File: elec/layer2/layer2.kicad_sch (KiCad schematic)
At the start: 19 parts

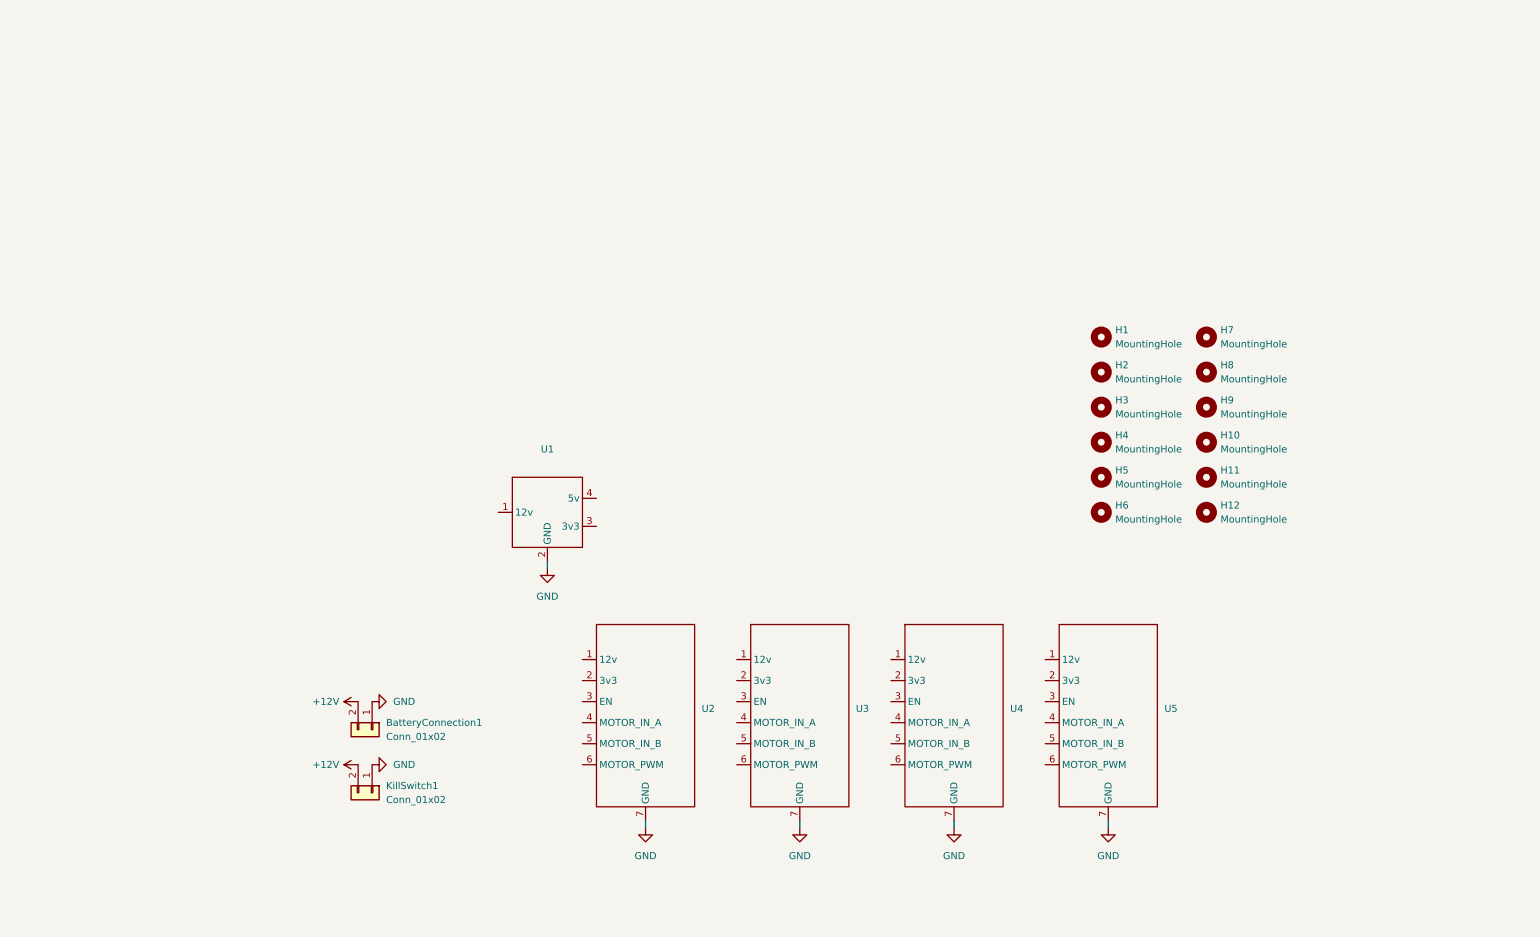
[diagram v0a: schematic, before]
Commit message: did some stuff on l2
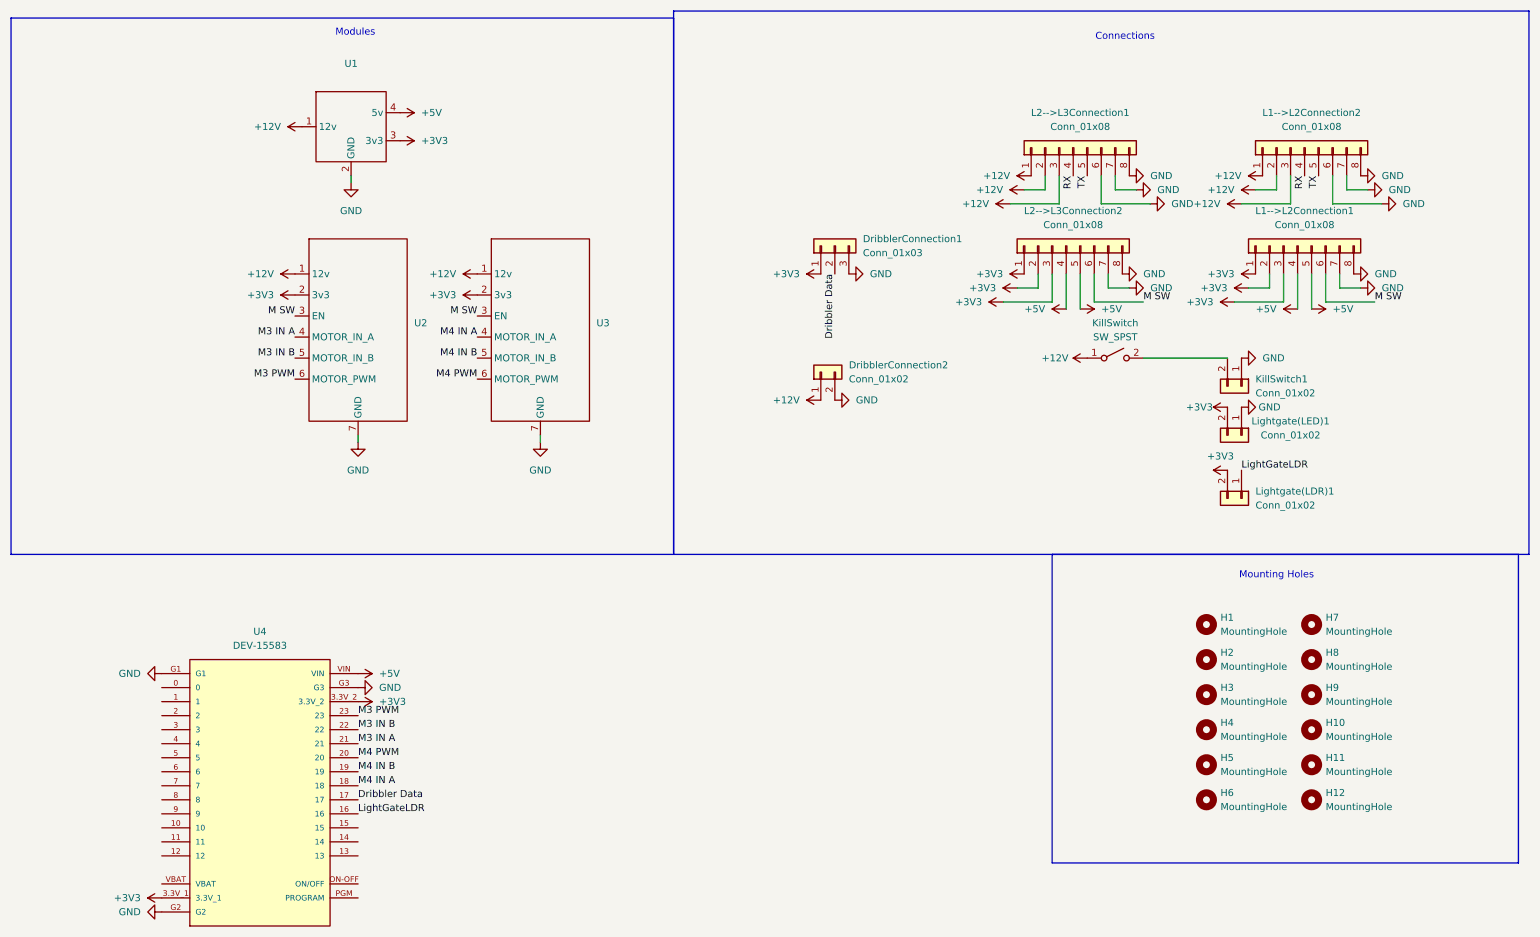
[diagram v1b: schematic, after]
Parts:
- removed BatteryConnection1: Conn_01x02, layer2-pcb-footprints:AMASS_XT60-M, symbol Connector_Generic:Conn_01x02
- removed U4, U5: ~, layer2-pcb-footprints:motor-driver-module, symbol layer2-pcb-symbols:motor-driver-module
- added DribblerConnection1: Conn_01x03, Pinheaders:PinHeader_1x03_P2.54mm_Vertical, symbol Connector_Generic:Conn_01x03
- added DribblerConnection2: Conn_01x02, Connector_AMASS:AMASS_XT30U-F_1x02_P5.0mm_Vertical, symbol Connector_Generic:Conn_01x02
- added KillSwitch: SW_SPST, Connector_AMASS:AMASS_XT30PW-M_1x02_P2.50mm_Horizontal, symbol Switch:SW_SPST
- added L1-->L2Connection1, L1-->L2Connection2, L2-->L3Connection1, L2-->L3Connection2: Conn_01x08, Pinheaders:PinHeader_1x08_P2.54mm_Vertical, symbol Connector_Generic:Conn_01x08
- added Lightgate(LDR)1, Lightgate(LED)1: Conn_01x02, Connector_JST:JST_SH_BM02B-SRSS-TB_1x02-1MP_P1.00mm_Vertical, symbol Connector_Generic:Conn_01x02
- added U4: DEV-15583, layer2-pcb-footprints:MODULE_DEV-15583, symbol Teensy4.0:DEV-15583
- KillSwitch1: footprint layer2-pcb-footprints:AMASS_XT60-M -> Connector_AMASS:AMASS_XT30U-F_1x02_P5.0mm_Vertical
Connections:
- net +12V: now also U1.1 (12v), U2.1 (12v), U3.1 (12v), DribblerConnection2.1 (Pin_1), KillSwitch.1 (A), L1-->L2Connection2.1 (Pin_1), L1-->L2Connection2.2 (Pin_2), L1-->L2Connection2.3 (Pin_3), L2-->L3Connection1.1 (Pin_1), L2-->L3Connection1.2 (Pin_2), L2-->L3Connection1.3 (Pin_3); no longer KillSwitch1.2 (Pin_2)
- net GND: now also DribblerConnection1.3 (Pin_3), DribblerConnection2.2 (Pin_2), L1-->L2Connection1.7 (Pin_7), L1-->L2Connection1.8 (Pin_8), L1-->L2Connection2.6 (Pin_6), L1-->L2Connection2.7 (Pin_7), L1-->L2Connection2.8 (Pin_8), L2-->L3Connection1.6 (Pin_6), L2-->L3Connection1.7 (Pin_7), L2-->L3Connection1.8 (Pin_8), L2-->L3Connection2.7 (Pin_7), L2-->L3Connection2.8 (Pin_8), Lightgate(LED)1.1 (Pin_1), U4.G1, U4.G2, U4.G3
- net +3V3: now reaches U1.3 (3v3)
- net +3V3: now also U2.2 (3v3), U3.2 (3v3), DribblerConnection1.1 (Pin_1), L1-->L2Connection1.1 (Pin_1), L1-->L2Connection1.2 (Pin_2), L1-->L2Connection1.3 (Pin_3), L2-->L3Connection2.1 (Pin_1), L2-->L3Connection2.2 (Pin_2), L2-->L3Connection2.3 (Pin_3), Lightgate(LDR)1.2 (Pin_2), Lightgate(LED)1.2 (Pin_2), U4.3.3V_1, U4.3.3V_2
- net +5V: now reaches U1.4 (5v)
- net +5V: now also L1-->L2Connection1.4 (Pin_4), L1-->L2Connection1.5 (Pin_5), L2-->L3Connection2.4 (Pin_4), L2-->L3Connection2.5 (Pin_5), U4.VIN
- net M SW: now reaches U3.3 (EN)
- net M SW: now also U2.3 (EN), L1-->L2Connection1.6 (Pin_6), L2-->L3Connection2.6 (Pin_6)
- net M4 IN A: now reaches U3.4 (MOTOR_IN_A)
- net M4 IN A: now also U4.18
- net M4 IN B: now reaches U3.5 (MOTOR_IN_B)
- net M4 IN B: now also U4.19
- net M4 PWM: now reaches U3.6 (MOTOR_PWM)
- net M4 PWM: now also U4.20
- net M3 IN A: now reaches U2.4 (MOTOR_IN_A)
- net M3 IN A: now also U4.21
- net M3 IN B: now reaches U2.5 (MOTOR_IN_B)
- net M3 IN B: now also U4.22
- net M3 PWM: now reaches U2.6 (MOTOR_PWM)
- net M3 PWM: now also U4.23
- new net: KillSwitch.2 (B), KillSwitch1.2 (Pin_2)
- new net Dribbler Data: DribblerConnection1.2 (Pin_2), U4.17
- new net LightGateLDR: Lightgate(LDR)1.1 (Pin_1), U4.16
- new net RX: L1-->L2Connection2.4 (Pin_4), L2-->L3Connection1.4 (Pin_4)
- new net TX: L1-->L2Connection2.5 (Pin_5), L2-->L3Connection1.5 (Pin_5)
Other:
- note added: "Connections"
- note added: "Modules"
- note added: "Mounting Holes"
- moved on the sheet: H1, H10, H11, H12, H2, H3, H4, H5, H6, H7, H8, H9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

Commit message: did something
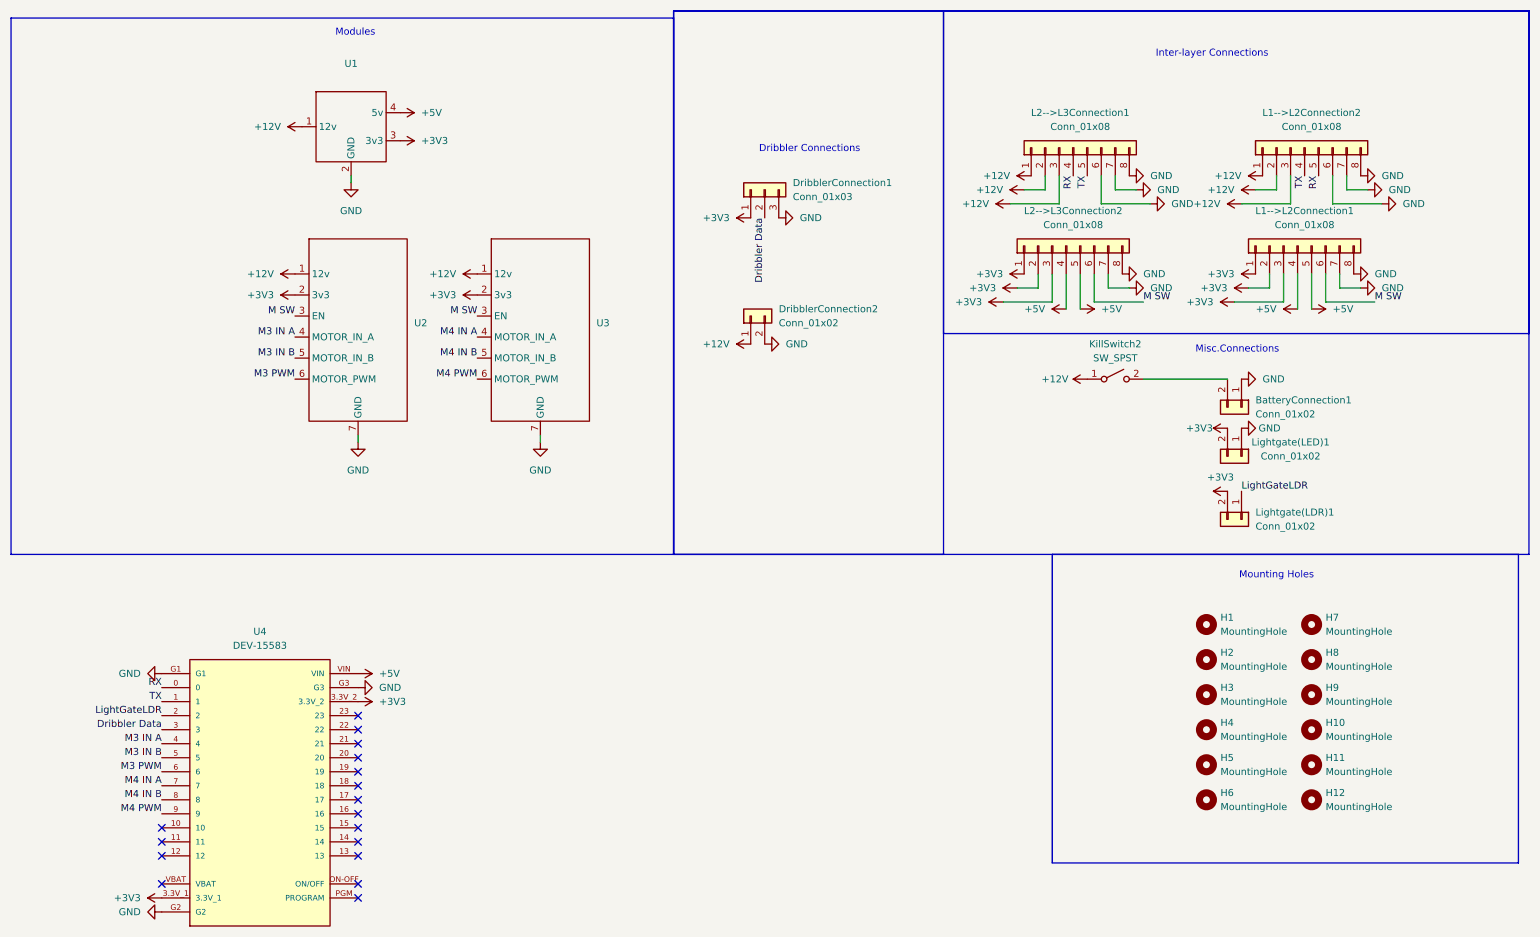
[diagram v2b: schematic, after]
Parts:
- KillSwitch2: renamed from KillSwitch; footprint Connector_AMASS:AMASS_XT30PW-M_1x02_P2.50mm_Horizontal -> Connector_AMASS:AMASS_XT30U-F_1x02_P5.0mm_Vertical
- renumbered KillSwitch1 to BatteryConnection1
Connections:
- net Dribbler Data: now also U4.3; no longer U4.17
- net LightGateLDR: now also U4.2; no longer U4.16
- net M3 IN A: now also U4.4; no longer U4.21
- net M3 IN B: now also U4.5; no longer U4.22
- net M3 PWM: now also U4.6; no longer U4.23
- net M4 IN A: now also U4.7; no longer U4.18
- net M4 IN B: now also U4.8; no longer U4.19
- net M4 PWM: now also U4.9; no longer U4.20
- net RX: now also L1-->L2Connection2.5 (Pin_5), U4.0; no longer L1-->L2Connection2.4 (Pin_4)
- net TX: now also L1-->L2Connection2.4 (Pin_4), U4.1; no longer L1-->L2Connection2.5 (Pin_5)
- no-connect marks 0 -> 17
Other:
- note added: "Dribbler Connections"
- note added: "Inter-layer Connections"
- note added: "Misc.Connections"
- note removed: "Connections"
- moved on the sheet: BatteryConnection1, DribblerConnection1, DribblerConnection2, KillSwitch2, Lightgate(LDR)1, Lightgate(LED)1

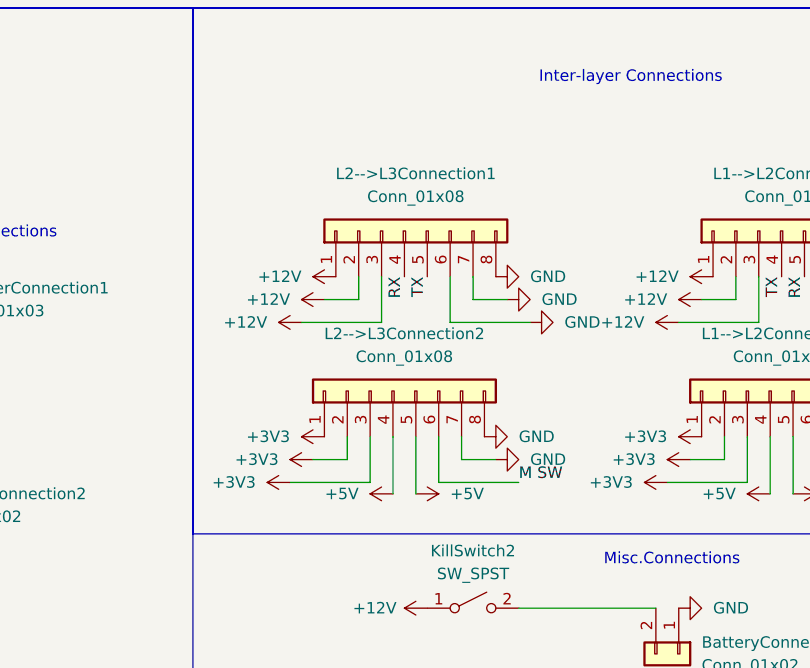
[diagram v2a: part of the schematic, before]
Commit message: did smnth to l2
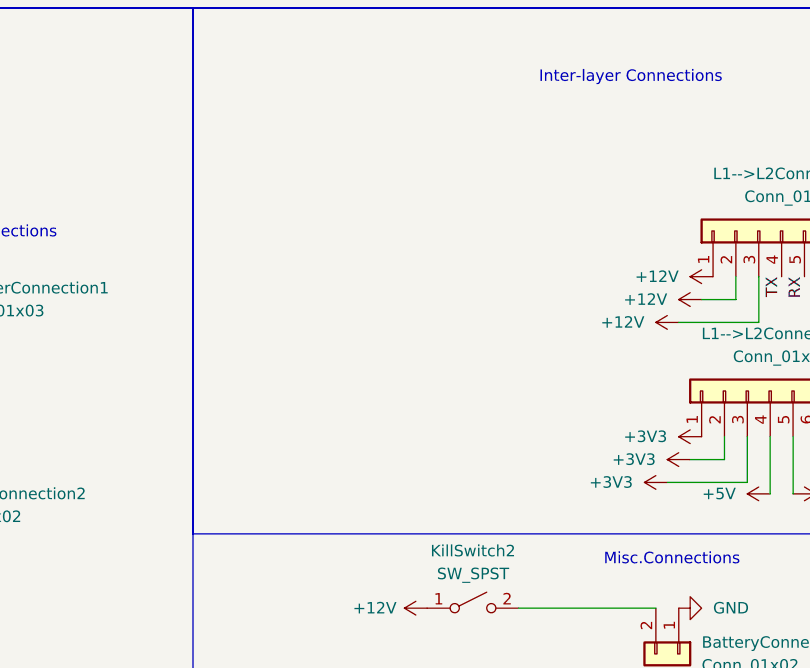
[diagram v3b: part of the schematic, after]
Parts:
- removed L2-->L3Connection1, L2-->L3Connection2: Conn_01x08, Pinheaders:PinHeader_1x08_P2.54mm_Vertical, symbol Connector_Generic:Conn_01x08
